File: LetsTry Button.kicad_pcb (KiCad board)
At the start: 2 copper layers, 51.8 x 124.5 mm, 36 parts, among them J1 Screw_Terminal_01x02, J2 Screw_Terminal_01x02, J3 Screw_Terminal_01x03, J4 1658525-8, J9 Screw_Terminal_01x02, P2 RB1-125BAG1A, P3 USB_C_Plug, U1 W5100, U2 ESP32-S3-DEVKITC-1-N8R2

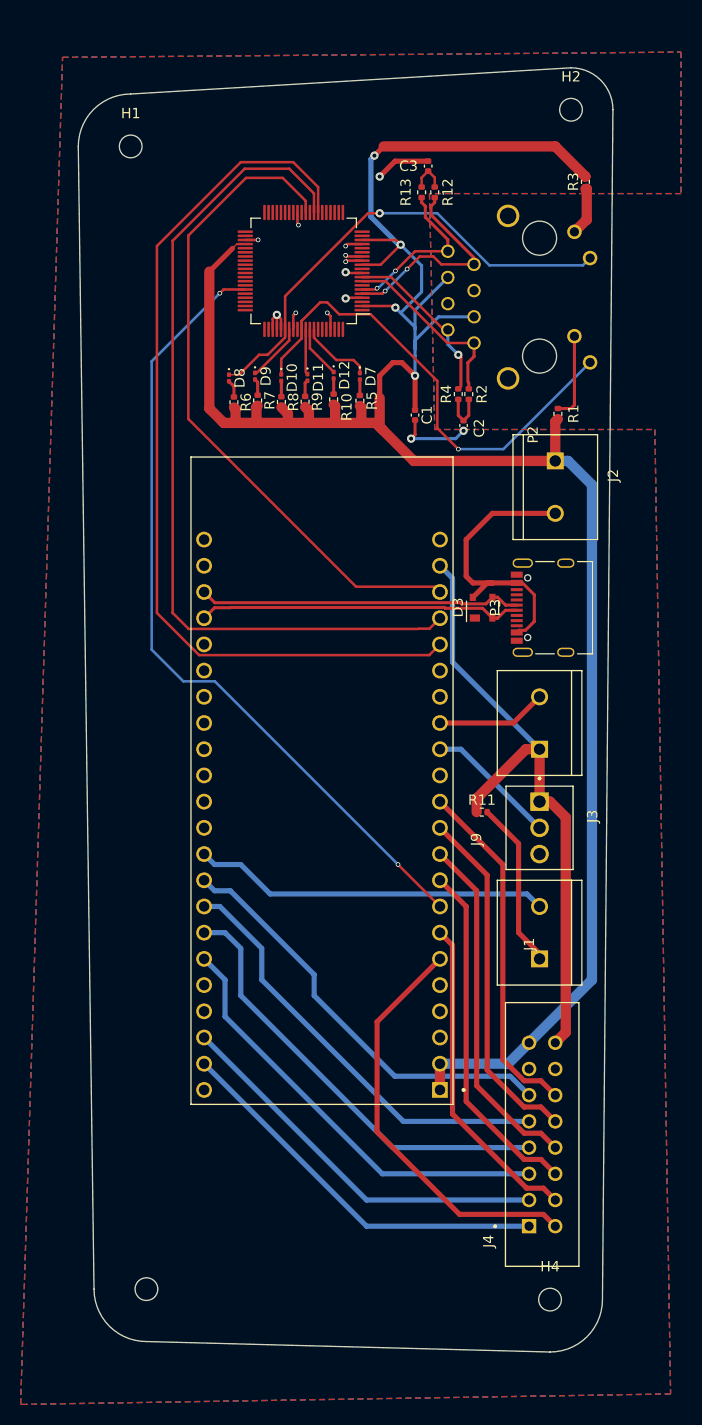
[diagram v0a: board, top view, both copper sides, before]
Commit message: Add files via upload
even new
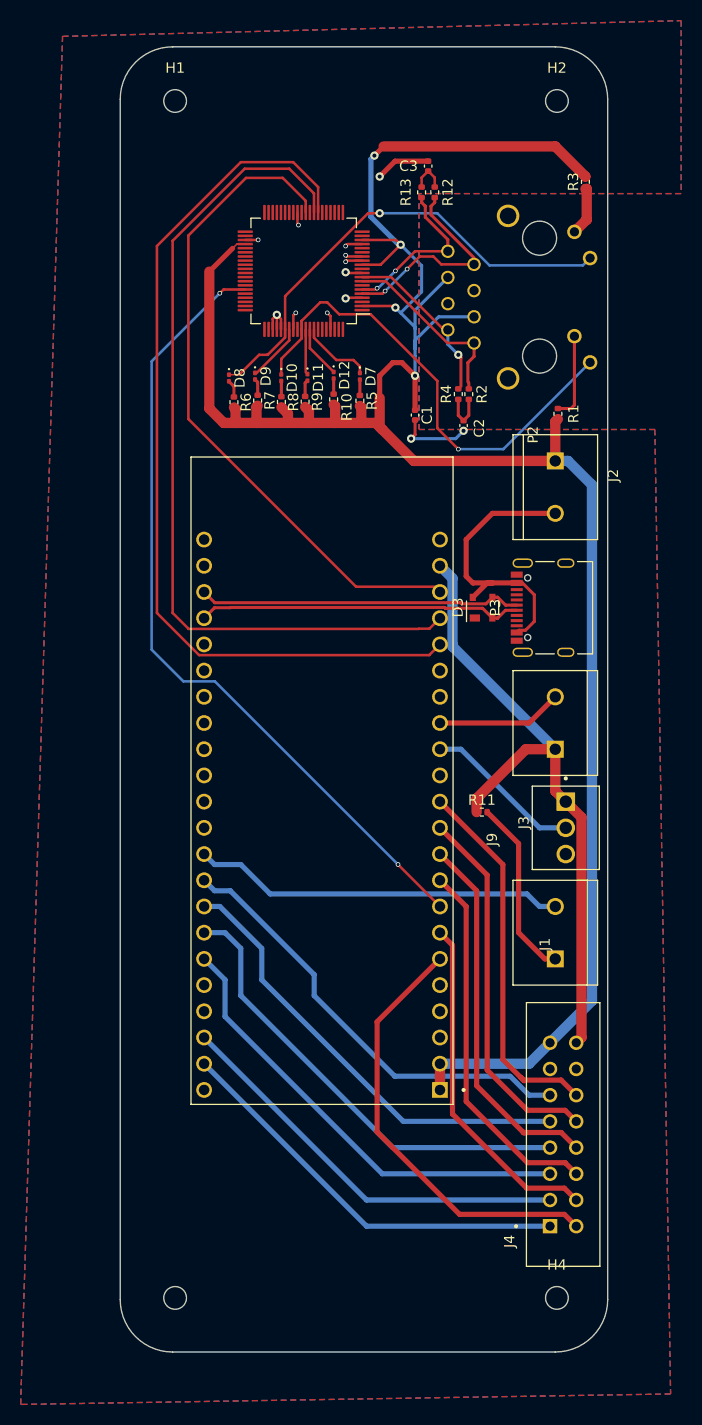
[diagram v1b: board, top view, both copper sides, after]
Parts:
- moved H1 6.16 mm to (112.0, 53.0)
- moved H3 2.91 mm to (112.0, 169.0)
- moved J3 2.54 mm to (149.9, 123.4)
- moved J4 2.03 mm to (149.6, 153.2)
- moved H2 1.61 mm to (149.0, 53.0)
- moved J1 1.52 mm to (148.8, 133.6)
- moved J9 1.52 mm to (148.8, 113.3)
- moved H4 0.68 mm to (149.0, 169.0)
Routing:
- net /W5100/GPIO46: track 12.8 -> 15.3 mm
- net /W5100/GPIO8: track 34.0 -> 36.5 mm
- net /W5100/GPIO17: track 34.0 -> 36.2 mm
- net /W5100/GPIO42: track 42.2 -> 44.2 mm
- net /W5100/GPIO16: track 34.0 -> 36.1 mm
- net /W5100/GPIO7: track 31.5 -> 33.5 mm
- net /W5100/GPIO6: track 40.3 -> 42.4 mm
- net /W5100/GPIO44: track 38.0 -> 40.1 mm
- net /W5100/GPIO43: track 38.0 -> 40.1 mm
- net /W5100/GPIO41: track 42.8 -> 44.8 mm
- net /W5100/GPIO40: track 41.9 -> 43.9 mm
- net /W5100/GPIO39: track 41.3 -> 43.3 mm
- net /W5100/GPIO18: track 34.0 -> 36.1 mm
- net Net-(J1-Pin_2): track 34.6 -> 36.1 mm
- net /W5100/GPIO9: track 10.7 -> 12.2 mm
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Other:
- board size 51.8 x 124.5 mm -> 47.2 x 126.5 mm
